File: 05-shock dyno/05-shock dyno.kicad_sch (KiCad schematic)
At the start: 15 parts, among them J1 Conn_01x03, J2 RJ45, J3 XT30PW-M, J4 Conn_01x04, U1 Teensy4.1

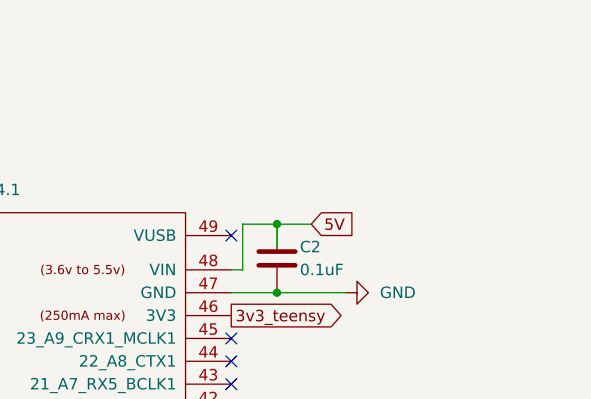
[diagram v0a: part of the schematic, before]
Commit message: v2 layout
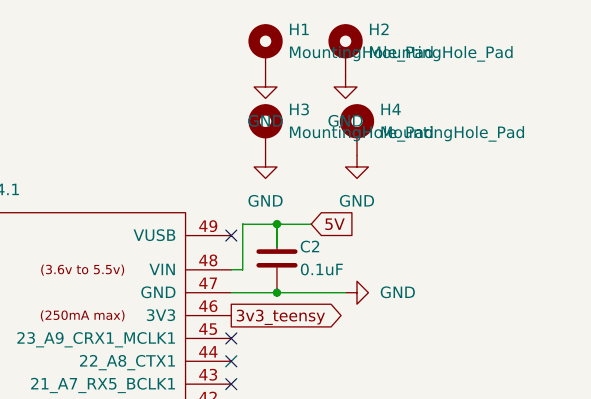
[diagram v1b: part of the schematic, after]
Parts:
- added H1, H2, H3, H4: MountingHole_Pad, MountingHole:MountingHole_4.3mm_M4, symbol Mechanical:MountingHole_Pad
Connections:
- net GND: now also H1.1, H2.1, H3.1, H4.1

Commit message: fixes
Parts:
- H1, H2, H3, H4: footprint MountingHole:MountingHole_4.3mm_M4 -> MountingHole:MountingHole_4.3mm_M4_DIN965_Pad
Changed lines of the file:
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@@
 			)
 		)
-		(property "Footprint" "MountingHole:MountingHole_4.3mm_M4"
+		(property "Footprint" "MountingHole:MountingHole_4.3mm_M4_DIN965_Pad"
 			(at 248.92 26.67 0)
 			(effects
@@
 			)
 		)
-		(property "Footprint" "MountingHole:MountingHole_4.3mm_M4"
+		(property "Footprint" "MountingHole:MountingHole_4.3mm_M4_DIN965_Pad"
 			(at 240.03 26.67 0)
 			(effects
@@
 			)
 		)
-		(property "Footprint" "MountingHole:MountingHole_4.3mm_M4"
+		(property "Footprint" "MountingHole:MountingHole_4.3mm_M4_DIN965_Pad"
 			(at 250.19 35.56 0)
 			(effects
@@
 			)
 		)
-		(property "Footprint" "MountingHole:MountingHole_4.3mm_M4"
+		(property "Footprint" "MountingHole:MountingHole_4.3mm_M4_DIN965_Pad"
 			(at 240.03 35.56 0)
 			(effects
